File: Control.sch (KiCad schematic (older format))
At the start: 22 parts, among them J10 LCD Header, J11 CONN_02X08, J8 JUMPER, J9 JUMPER, U10 MB85RC256V, U5 Teensy_3.2_NoProg, U6 REF2041, U7 DAC121C085, U8 DAC121C085, U9 ADS1115

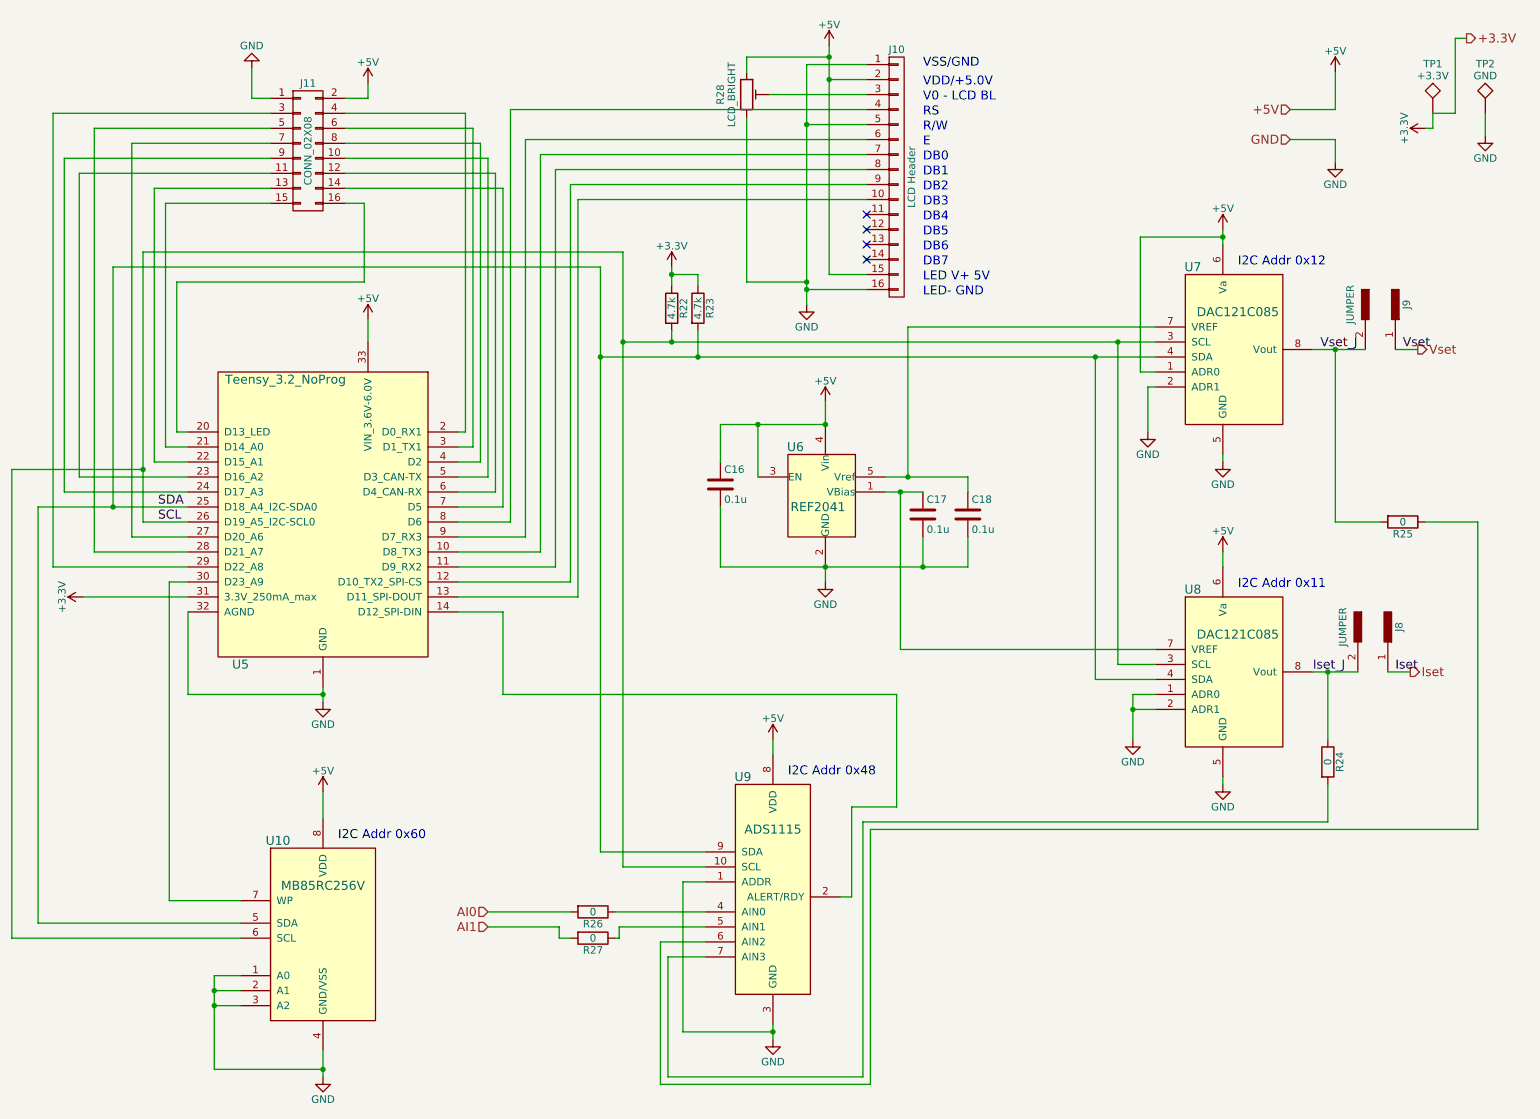
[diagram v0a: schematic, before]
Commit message: Finished routing
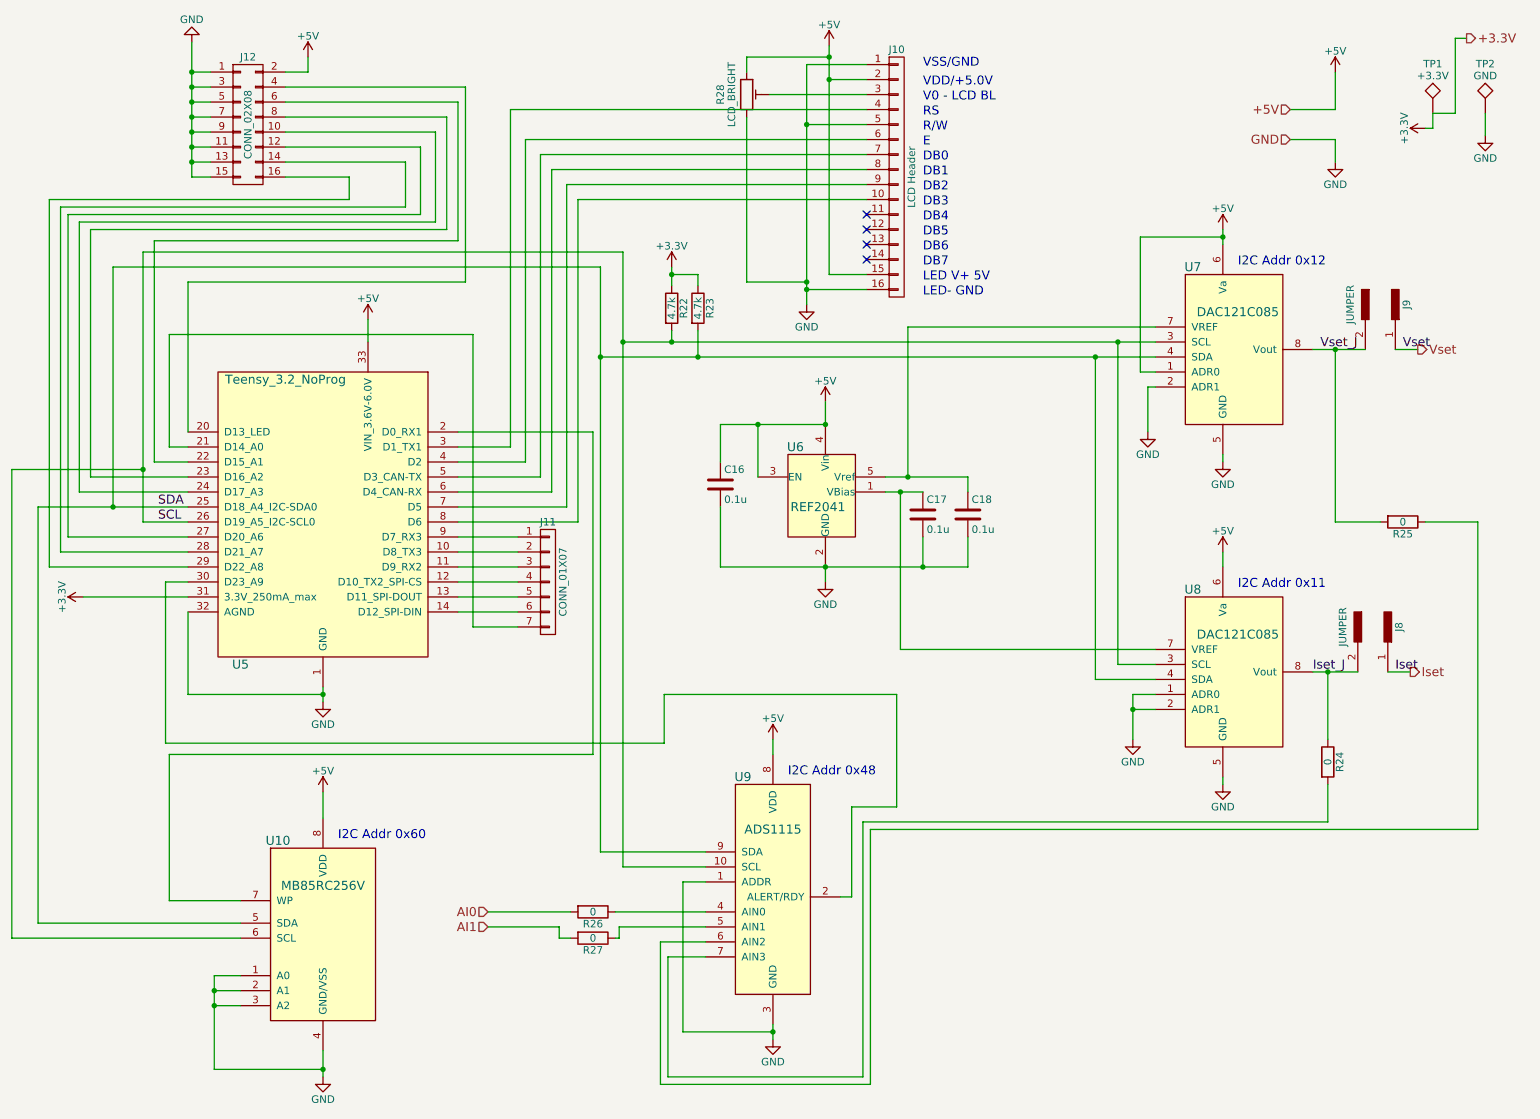
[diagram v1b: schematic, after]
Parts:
- removed J11: CONN_02X08, Connectors:IDC_Header_Straight_16pins, symbol CONN_02X08
- added J11: CONN_01X07, Pin_Headers:Pin_Header_Straight_1x07_Pitch2.54mm, symbol CONN_01X07
- added J12: CONN_02X08, Connectors:IDC_Header_Straight_16pins, symbol CONN_02X08
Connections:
- net +5V: now also J12.2 (P2)
- net GND: now also J12.1 (P1), J12.11 (P11), J12.13 (P13), J12.15 (P15), J12.3 (P3), J12.5 (P5), J12.7 (P7), J12.9 (P9)
- net at U5.10 (D8_TX3): now also J11.2 (P2); no longer J10.7 (P7)
- net at U5.11 (D9_RX2): now also J11.3 (P3); no longer J10.8 (P8)
- net at U5.12 (D10_TX2_SPI-CS): now also J11.4 (P4); no longer J10.9 (P9)
- net at U5.13 (D11_SPI-DOUT): now also J11.5 (P5); no longer J10.10 (P10)
- net at U5.14 (D12_SPI-DIN): now also J11.6 (P6); no longer U9.2 (ALERT/RDY)
- net at U5.2 (D0_RX1): now also U10.7 (WP)
- net at U5.20 (D13_LED): now also J12.4 (P4)
- net at U5.21 (D14_A0): now also J11.7 (P7)
- net at U5.22 (D15_A1): now also J12.6 (P6)
- net at U5.23 (D16_A2): now also J12.8 (P8)
- net at U5.24 (D17_A3): now also J12.10 (P10)
- net at U5.27 (D20_A6): now also J12.12 (P12)
- net at U5.28 (D21_A7): now also J12.14 (P14)
- net at U5.29 (D22_A8): now also J12.16 (P16)
- net at U5.3 (D1_TX1): now also J10.4 (P4)
- net at U5.30 (D23_A9): now also U9.2 (ALERT/RDY); no longer U10.7 (WP)
- net at U5.4 (D2): now also J10.6 (P6)
- net at U5.5 (D3_CAN-TX): now also J10.7 (P7)
- net at U5.6 (D4_CAN-RX): now also J10.8 (P8)
- net at U5.7 (D5): now also J10.9 (P9)
- net at U5.8 (D6): now also J10.10 (P10); no longer J10.4 (P4)
- net at U5.9 (D7_RX3): now also J11.1 (P1); no longer J10.6 (P6)
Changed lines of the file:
@@
-$EndComp
-$Comp
-L CONN_02X08 J11
-U 1 1 591E21F8
-P 2800 1375
-F 0 "J11" H 2800 1825 50  0000 C CNN
-F 1 "CONN_02X08" V 2800 1375 50  0000 C CNN
-F 2 "Connectors:IDC_Header_Straight_16pins" H 2800 175 50  0001 C CNN
-F 3 "" H 2800 175 50  0001 C CNN
-	1    2800 1375
-	1    0    0    -1
 $EndComp
 $Comp
 L +5V #PWR087
 U 1 1 591E25DD
-P 3200 925
-F 0 "#PWR087" H 3200 775 50  0001 C CNN
-F 1 "+5V" H 3200 1065 50  0000 C CNN
-F 2 "" H 3200 925 50  0001 C CNN
-F 3 "" H 3200 925 50  0001 C CNN
-	1    3200 925
+P 2800 750
+F 0 "#PWR087" H 2800 600 50  0001 C CNN
+F 1 "+5V" H 2800 890 50  0000 C CNN
+F 2 "" H 2800 750 50  0001 C CNN
+F 3 "" H 2800 750 50  0001 C CNN
+	1    2800 750
 	1    0    0    -1
 $EndComp
@@
 L GND #PWR088
 U 1 1 591E262A
-P 2425 825
-F 0 "#PWR088" H 2425 575 50  0001 C CNN
-F 1 "GND" H 2425 675 50  0000 C CNN
-F 2 "" H 2425 825 50  0001 C CNN
-F 3 "" H 2425 825 50  0001 C CNN
-	1    2425 825
+P 2025 650
+F 0 "#PWR088" H 2025 400 50  0001 C CNN
+F 1 "GND" H 2025 500 50  0000 C CNN
+F 2 "" H 2025 650 50  0001 C CNN
+F 3 "" H 2025 650 50  0001 C CNN
+	1    2025 650
 	-1   0    0    1
 $EndComp
@@
 Connection ~ 5800 3200
 Wire Wire Line
-	6250 3050 6250 3200
+	6250 3200 6250 3050
 Wire Wire Line
 	6650 3550 7200 3550
@@
 Wire Wire Line
 	8050 4900 8450 4900
-Wire Wire Line
-	1700 2050 1700 3850
 Wire Wire Line
 	1700 2050 4900 2050
@@
 	6725 5750 6725 5000
 Wire Wire Line
-	6725 5000 4100 5000
-Wire Wire Line
-	4100 5000 4100 4450
-Wire Wire Line
-	4100 4450 3800 4450
-Wire Wire Line
 	5450 6450 4850 6450
 Wire Wire Line
@@
 	1875 6375 2350 6375
 Wire Wire Line
-	1875 6375 1875 4250
-Wire Wire Line
-	1875 4250 2000 4250
-Wire Wire Line
 	6525 800  6125 800
 Wire Wire Line
@@
 Connection ~ 6125 1200
 Wire Wire Line
-	3800 4350 4600 4350
-Wire Wire Line
-	4600 4350 4600 1700
-Wire Wire Line
 	4600 1700 6525 1700
 Wire Wire Line
-	6525 1600 4550 1600
-Wire Wire Line
-	4550 1600 4550 4250
-Wire Wire Line
-	4550 4250 3800 4250
-Wire Wire Line
-	3800 4150 4450 4150
-Wire Wire Line
-	4450 4150 4450 1500
-Wire Wire Line
-	4450 1500 6525 1500
+	4525 1600 6525 1600
+Wire Wire Line
+	4425 1500 6525 1500
 Wire Wire Line
 	6525 1400 4350 1400
 Wire Wire Line
-	4350 1400 4350 4050
-Wire Wire Line
-	4350 4050 3800 4050
-Wire Wire Line
-	3800 3950 4250 3950
-Wire Wire Line
-	4250 3950 4250 1300
-Wire Wire Line
 	4250 1300 6525 1300
 Wire Wire Line
 	6525 1100 4150 1100
 Wire Wire Line
-	4150 1100 4150 3850
-Wire Wire Line
-	4150 3850 3800 3850
-Wire Wire Line
-	3200 925  3200 1025
-Wire Wire Line
-	3200 1025 3050 1025
-Wire Wire Line
-	2425 825  2425 1025
-Wire Wire Line
-	2425 1025 2550 1025
-Wire Wire Line
-	3800 3250 3850 3250
-Wire Wire Line
-	3850 3250 3850 1125
-Wire Wire Line
-	3850 1125 3050 1125
-Wire Wire Line
-	3800 3350 3900 3350
-Wire Wire Line
-	3900 3350 3900 1225
-Wire Wire Line
-	3900 1225 3050 1225
-Wire Wire Line
-	3800 3450 3950 3450
-Wire Wire Line
-	3950 3450 3950 1325
-Wire Wire Line
-	3950 1325 3050 1325
-Wire Wire Line
-	3800 3550 4000 3550
-Wire Wire Line
-	4000 3550 4000 1425
-Wire Wire Line
-	4000 1425 3050 1425
-Wire Wire Line
-	3800 3650 4050 3650
-Wire Wire Line
-	4050 3650 4050 1525
-Wire Wire Line
-	4050 1525 3050 1525
-Wire Wire Line
-	3800 3750 4100 3750
-Wire Wire Line
-	4100 3750 4100 1625
-Wire Wire Line
-	4100 1625 3050 1625
-Wire Wire Line
-	3050 1725 3175 1725
-Wire Wire Line
-	3175 1725 3175 2250
-Wire Wire Line
-	3175 2250 1925 2250
-Wire Wire Line
-	1925 2250 1925 3250
-Wire Wire Line
-	1925 3250 2000 3250
-Wire Wire Line
-	2000 3350 1850 3350
-Wire Wire Line
-	1850 3350 1850 1725
-Wire Wire Line
-	1850 1725 2550 1725
-Wire Wire Line
-	2000 3450 1775 3450
-Wire Wire Line
-	1775 3450 1775 1625
-Wire Wire Line
-	1775 1625 2550 1625
-Wire Wire Line
-	2000 3550 1275 3550
-Wire Wire Line
-	1275 3550 1275 1525
-Wire Wire Line
-	1275 1525 2550 1525
-Wire Wire Line
-	1175 3650 2000 3650
-Wire Wire Line
-	1175 3650 1175 1425
-Wire Wire Line
-	1175 1425 2550 1425
+	2800 750  2800 850
+Wire Wire Line
+	2800 850  2650 850
+Wire Wire Line
+	2025 650  2025 1550
+Wire Wire Line
+	2025 850  2150 850
 Wire Wire Line
 	1500 2150 1500 3750
@@
 Connection ~ 5225 2200
 Wire Wire Line
-	1625 3950 2000 3950
-Wire Wire Line
-	1625 3950 1625 1325
-Wire Wire Line
-	1625 1325 2550 1325
-Wire Wire Line
-	2550 1225 1375 1225
-Wire Wire Line
-	1375 1225 1375 4050
-Wire Wire Line
-	1375 4050 2000 4050
-Wire Wire Line
-	2000 4150 1100 4150
-Wire Wire Line
-	1100 4150 1100 1125
-Wire Wire Line
-	1100 1125 2550 1125
-Wire Wire Line
 	2000 4450 2000 5000
 Wire Wire Line
@@
 Connection ~ 6800 3550
 Wire Wire Line
-	6250 3200 5550 3200
+	5550 3200 6250 3200
+Wire Wire Line
+	1700 2050 1700 3850
+Wire Wire Line
+	6725 5000 5175 5000
+Wire Wire Line
+	1875 6375 1875 5400
+Wire Wire Line
+	1875 5400 4700 5400
+Wire Wire Line
+	4700 5400 4700 3250
+Wire Wire Line
+	4700 3250 3800 3250
+$Comp
+L CONN_01X07 J11
+U 1 1 591E7FAC
+P 4400 4250
+F 0 "J11" H 4400 4650 50  0000 C CNN
+F 1 "CONN_01X07" V 4500 4250 50  0000 C CNN
+F 2 "Pin_Headers:Pin_Header_Straight_1x07_Pitch2.54mm" H 4400 4250 50  0001 C CNN
+F 3 "" H 4400 4250 50  0001 C CNN
+	1    4400 4250
+	1    0    0    -1
+$EndComp
+Wire Wire Line
+	4150 3350 3800 3350
+Wire Wire Line
+	4150 1100 4150 3350
+Wire Wire Line
+	3800 3450 4250 3450
+Wire Wire Line
+	3800 3550 4350 3550
+Wire Wire Line
+	3800 3650 4425 3650
+Wire Wire Line
+	3800 3750 4525 3750
+Wire Wire Line
+	3800 3850 4600 3850
+Wire Wire Line
+	4250 3450 4250 1300
+Wire Wire Line
+	4350 3550 4350 1400
+Wire Wire Line
+	4425 3650 4425 1500
+Wire Wire Line
+	4525 3750 4525 1600
+Wire Wire Line
+	4600 3850 4600 1700
+Wire Wire Line
+	5175 5000 5175 5325
+Wire Wire Line
+	5175 5325 1850 5325
+Wire Wire Line
+	1850 5325 1850 4250
+Wire Wire Line
+	1850 4250 2000 4250
+Wire Wire Line
+	3800 3950 4200 3950
+Wire Wire Line
+	3800 4050 4200 4050
+Wire Wire Line
+	4200 4150 3800 4150
+Wire Wire Line
+	3800 4250 4200 4250
+Wire Wire Line
+	4200 4350 3800 4350
+Wire Wire Line
+	3800 4450 4200 4450
+Wire Wire Line
+	1875 2600 1875 3350
+Wire Wire Line
+	1875 2600 3900 2600
+Wire Wire Line
+	3900 2600 3900 4550
+Wire Wire Line
+	3900 4550 4200 4550
+$Comp
+L CONN_02X08 J12
+U 1 1 591F25AB
+P 2400 1200
+F 0 "J12" H 2400 1650 50  0000 C CNN
+F 1 "CONN_02X08" V 2400 1200 50  0000 C CNN
+F 2 "Connectors:IDC_Header_Straight_16pins" H 2400 0   50  0001 C CNN
+F 3 "" H 2400 0   50  0001 C CNN
+	1    2400 1200
+	1    0    0    -1
+$EndComp
+Wire Wire Line
+	1875 3350 2000 3350
+Wire Wire Line
+	2025 1550 2150 1550
+Connection ~ 2025 850
+Wire Wire Line
+	2150 1450 2025 1450
+Connection ~ 2025 1450
+Wire Wire Line
+	2150 1350 2025 1350
+Connection ~ 2025 1350
+Wire Wire Line
+	2150 1250 2025 1250
+Connection ~ 2025 1250
+Wire Wire Line
+	2025 1150 2150 1150
+Connection ~ 2025 1150
+Wire Wire Line
+	2150 1050 2025 1050
+Connection ~ 2025 1050
+Wire Wire Line
+	2150 950  2025 950
+Connection ~ 2025 950
+Wire Wire Line
+	2650 950  3850 950
+Wire Wire Line
+	2000 3250 2000 2250
+Wire Wire Line
+	2000 2250 3850 2250
+Wire Wire Line
+	3850 2250 3850 950
+Wire Wire Line
+	2650 1050 3800 1050
+Wire Wire Line
+	2000 3450 1775 3450
+Wire Wire Line
+	1775 3450 1775 1975
+Wire Wire Line
+	1775 1975 3800 1975
+Wire Wire Line
+	3800 1975 3800 1050
+Wire Wire Line
+	2650 1150 3725 1150
+Wire Wire Line
+	2650 1250 3650 1250
+Wire Wire Line
+	3725 1150 3725 1900
+Wire Wire Line
+	3725 1900 1350 1900
+Wire Wire Line
+	1350 1900 1350 3550
+Wire Wire Line
+	1350 3550 2000 3550
+Wire Wire Line
+	2000 3650 1275 3650
+Wire Wire Line
+	1275 3650 1275 1850
+Wire Wire Line
+	1275 1850 3650 1850
+Wire Wire Line
+	3650 1850 3650 1250
+Wire Wire Line
+	2650 1350 3550 1350
+Wire Wire Line
+	2650 1450 3450 1450
+Wire Wire Line
+	3550 1350 3550 1800
+Wire Wire Line
+	3550 1800 1200 1800
+Wire Wire Line
+	1200 1800 1200 3950
+Wire Wire Line
+	1200 3950 2000 3950
+Wire Wire Line
+	3450 1450 3450 1750
+Wire Wire Line
+	3450 1750 1150 1750
+Wire Wire Line
+	1150 1750 1150 4050
+Wire Wire Line
+	1150 4050 2000 4050
+Wire Wire Line
+	2650 1550 3075 1550
+Wire Wire Line
+	3075 1550 3075 1700
+Wire Wire Line
+	3075 1700 1075 1700
+Wire Wire Line
+	1075 1700 1075 4150
+Wire Wire Line
+	1075 4150 2000 4150
 $EndSCHEMATC
